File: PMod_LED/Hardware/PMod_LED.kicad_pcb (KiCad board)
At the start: 2 copper layers, 25.5 x 60.2 mm, 83 parts, among them J1 Conn_02x06_Odd_Even, J2 Conn_02x06_Odd_Even, J3 Conn_02x06_Odd_Even

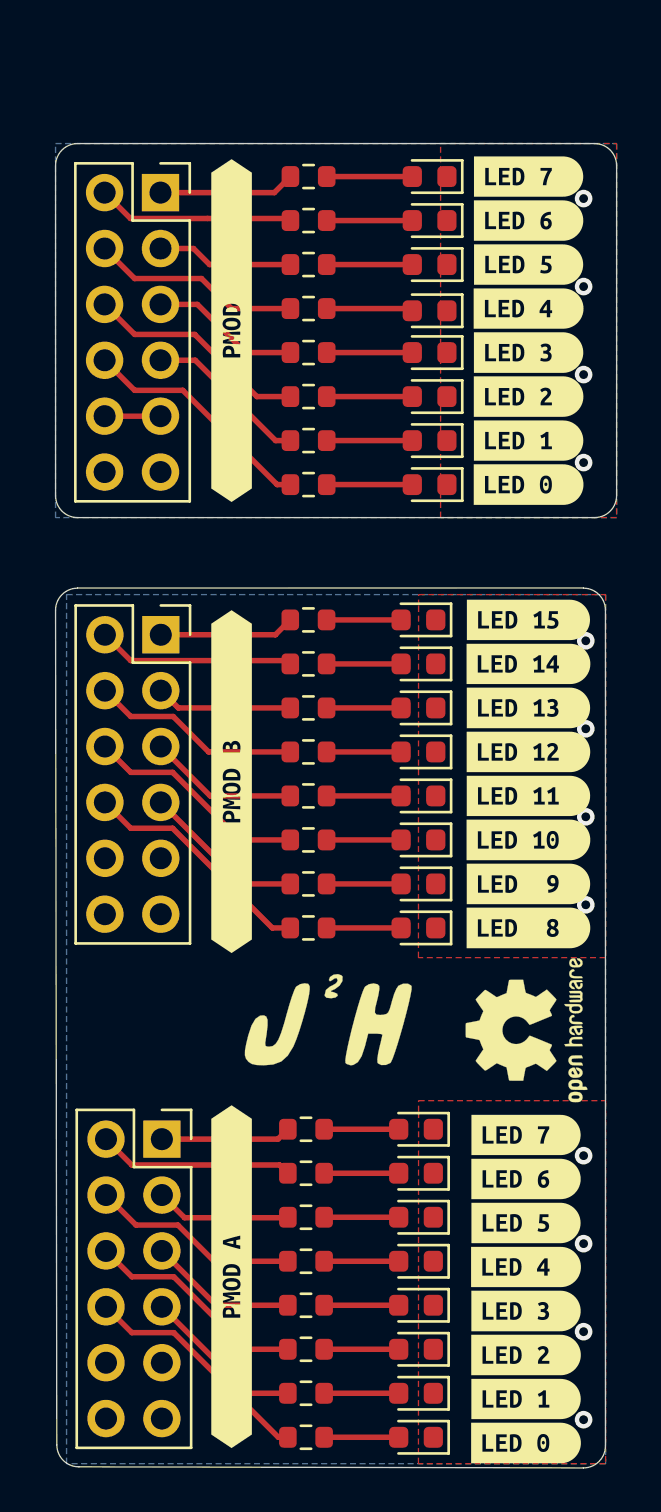
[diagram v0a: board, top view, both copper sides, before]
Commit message: Add join between the two PCB's
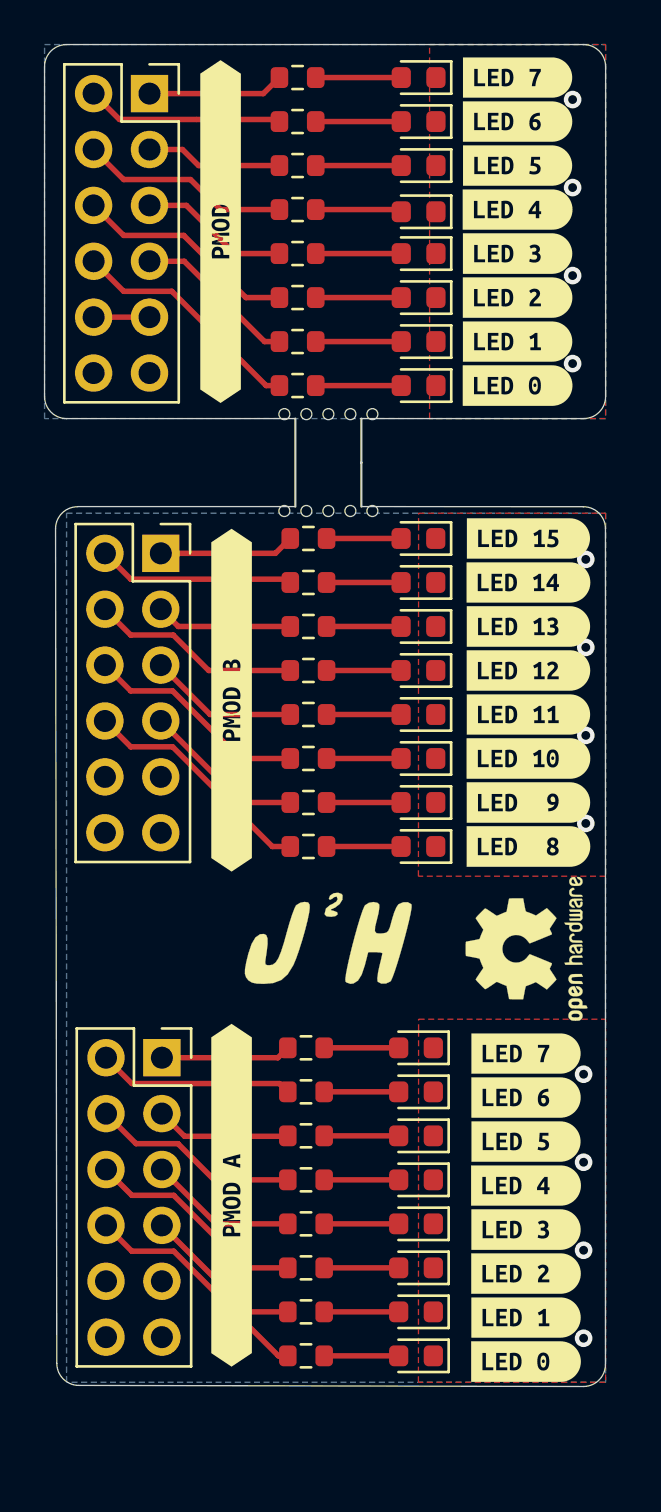
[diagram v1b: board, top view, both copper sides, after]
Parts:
- added REF**: NPTH, NPTH, F.Cu at (141.4, 95.2)
- added REF**: NPTH, NPTH, F.Cu at (140.4, 90.8)
- added REF**: NPTH, NPTH, F.Cu at (142.4, 90.8)
- added REF**: NPTH, NPTH, F.Cu at (141.4, 90.8)
- added REF**: NPTH, NPTH, F.Cu at (143.4, 90.8)
- added REF**: NPTH, NPTH, F.Cu at (142.4, 95.2)
- added REF**: NPTH, NPTH, F.Cu at (140.4, 95.2)
- added REF**: NPTH, NPTH, F.Cu at (144.4, 90.8)
- added REF**: NPTH, NPTH, F.Cu at (143.4, 95.2)
- added REF**: NPTH, NPTH, F.Cu at (144.4, 95.2)
- moved D1 4.53 mm to (146.5, 89.5)
- moved D2 4.53 mm to (146.5, 87.5)
- moved D3 4.53 mm to (146.5, 85.5)
- moved D4 4.53 mm to (146.5, 83.5)
- moved D5 4.53 mm to (146.5, 81.6)
- moved D6 4.53 mm to (146.5, 79.5)
- moved D7 4.53 mm to (146.5, 77.5)
- moved D8 4.53 mm to (146.5, 75.5)
- moved G*** 4.53 mm to (138.5, 82.2)
- moved J1 4.53 mm to (134.3, 76.2)
- moved R1 4.53 mm to (141.0, 89.5)
- moved R2 4.53 mm to (141.0, 87.5)
- moved R3 4.53 mm to (141.0, 85.5)
- moved R4 4.53 mm to (141.0, 83.5)
- moved R5 4.53 mm to (141.0, 81.5)
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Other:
- board size 25.5 x 60.2 mm -> 25.5 x 61 mm

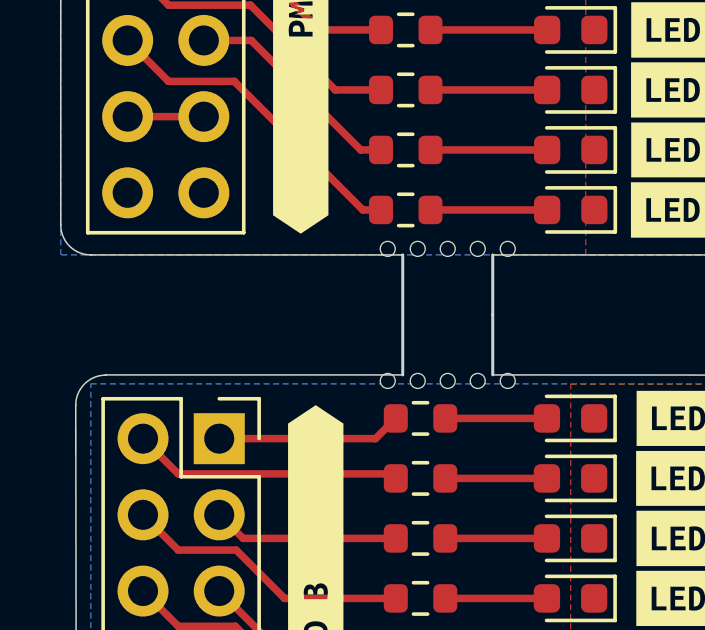
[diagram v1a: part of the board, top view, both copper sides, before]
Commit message: Fix the DRC errors on duel LED board
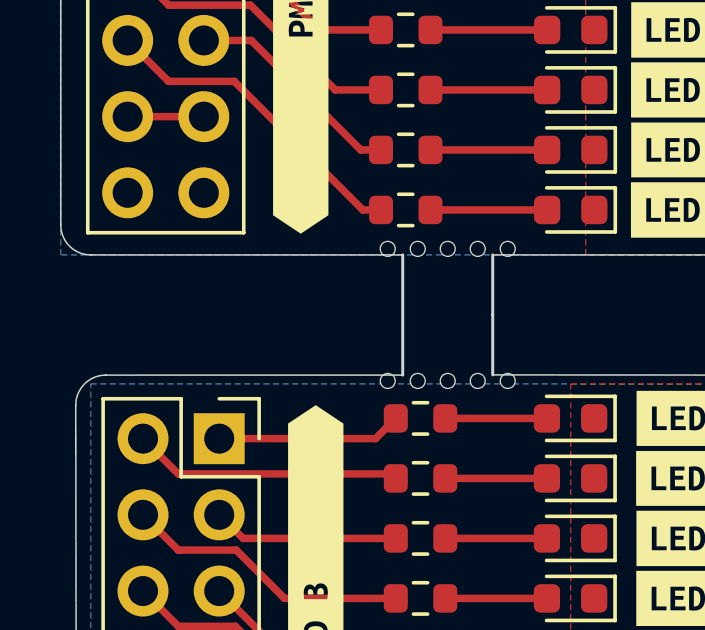
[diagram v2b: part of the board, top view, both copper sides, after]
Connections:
- D1 pad 1: GND -> GND2
- D2 pad 1: GND -> GND2
- D3 pad 1: GND -> GND2
- D4 pad 1: GND -> GND2
- D5 pad 1: GND -> GND2
- D6 pad 1: GND -> GND2
- D7 pad 1: GND -> GND2
- D8 pad 1: GND -> GND2
- J1 pad 10: GND -> GND2
- J1 pad 9: GND -> GND2
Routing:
- net GND2: track 0.00 -> 2.54 mm, vias 0 -> 4
- net GND: track 2.54 -> 0.00 mm, vias 12 -> 8
- added copper zone on B.Cu, net GND2
- added copper zone on F.Cu, net GND2
